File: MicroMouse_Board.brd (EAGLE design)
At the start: 129.2 x 106.7 mm, 64 parts

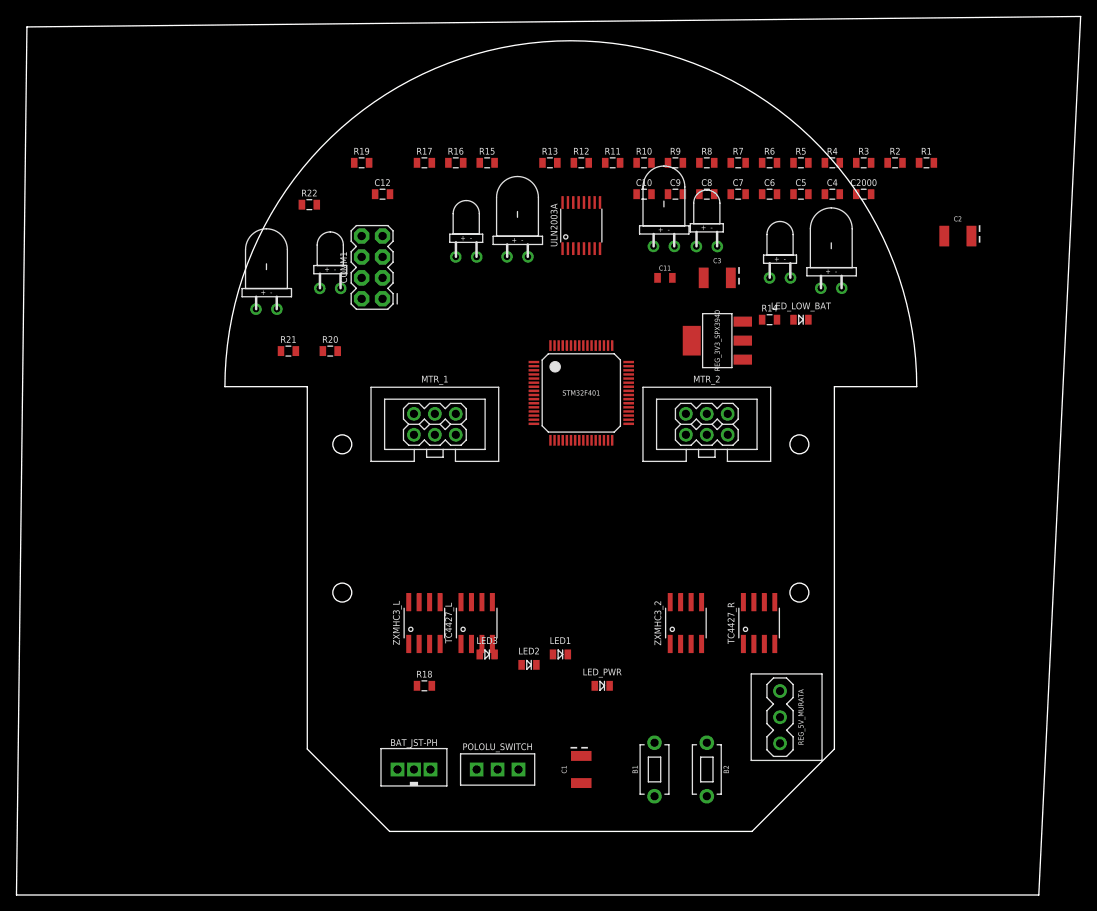
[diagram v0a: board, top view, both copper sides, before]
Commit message: Add files via upload
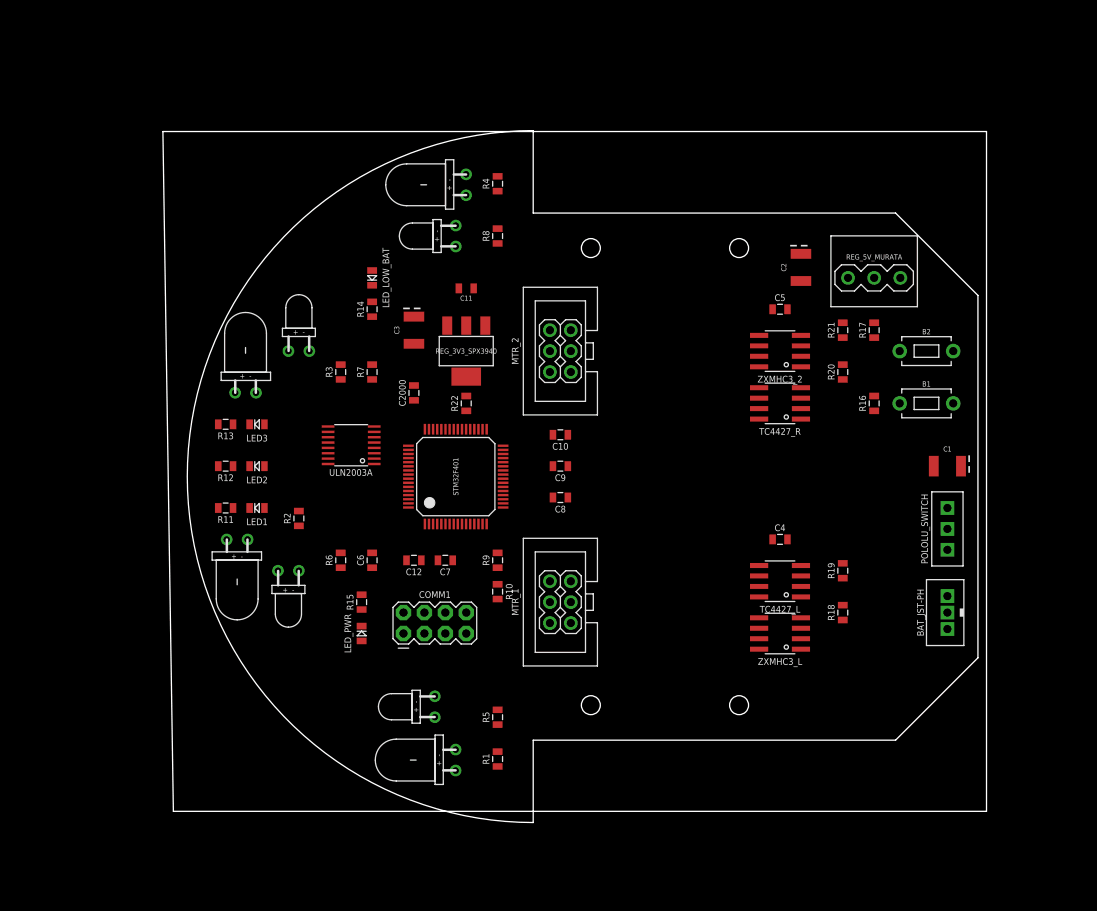
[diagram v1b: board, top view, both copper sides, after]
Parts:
- moved R1 89.2 mm to (39.4, 6.35), turned to 90 degrees
- moved R2 84.3 mm to (15.2, 35.6), turned to 90 degrees
- moved R5 76.7 mm to (39.4, 11.4), turned to 90 degrees
- moved R19 76.6 mm to (81.3, 29.2), turned to 90 degrees
- moved R6 71.0 mm to (20.3, 30.5), turned to 90 degrees
- moved RE_LD 69.5 mm to (14.0, 29.2), turned to 180 degrees
- moved R3 68.4 mm to (20.3, 53.3), turned to 90 degrees
- moved BAT_JST-PH 67.5 mm to (94.0, 24.1), turned to 90 degrees
- moved R21 67.4 mm to (81.3, 58.4), turned to 90 degrees
- moved EM_1 67.2 mm to (34.3, 6.35), turned to 90 degrees
- moved C6 65.6 mm to (24.1, 30.5), turned to 90 degrees
- moved RE_LF 64.9 mm to (31.8, 12.7), turned to 90 degrees
- moved R11 63.0 mm to (6.35, 36.8), turned to 180 degrees
- moved R20 62.3 mm to (81.3, 53.3), turned to 90 degrees
- moved POLOLU_SWITCH 61.9 mm to (94.0, 34.3), turned to 90 degrees
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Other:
- board size 129.2 x 106.7 mm -> 100 x 82.5 mm
